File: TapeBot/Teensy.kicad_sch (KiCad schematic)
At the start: 1 part

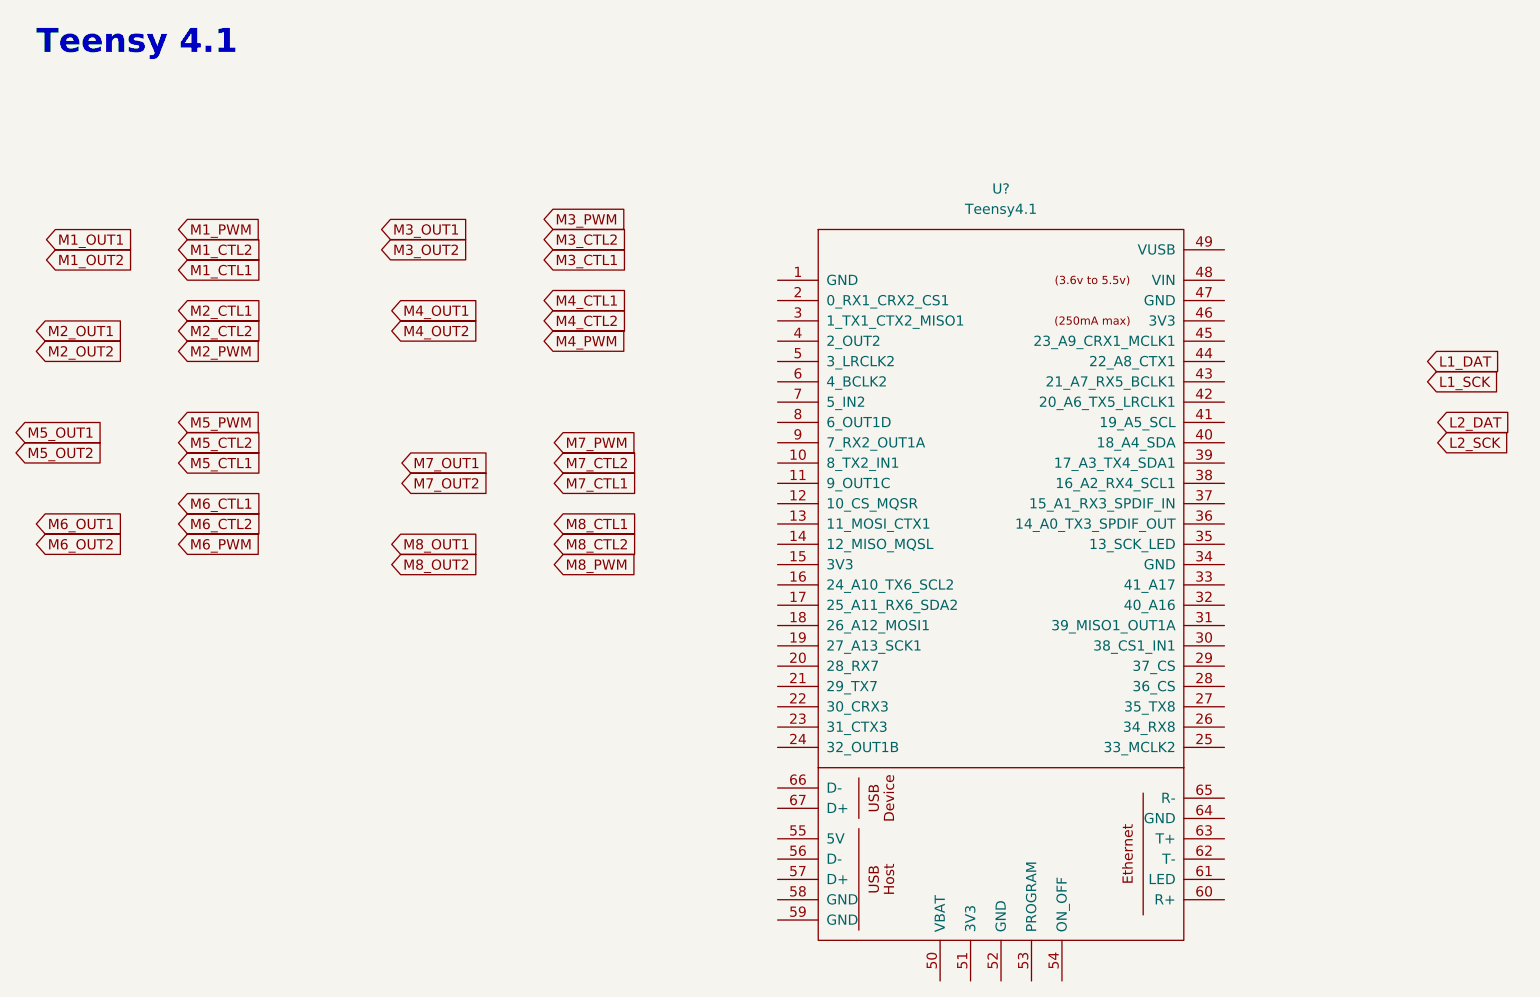
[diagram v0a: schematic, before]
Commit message: (mostly) finished schematic
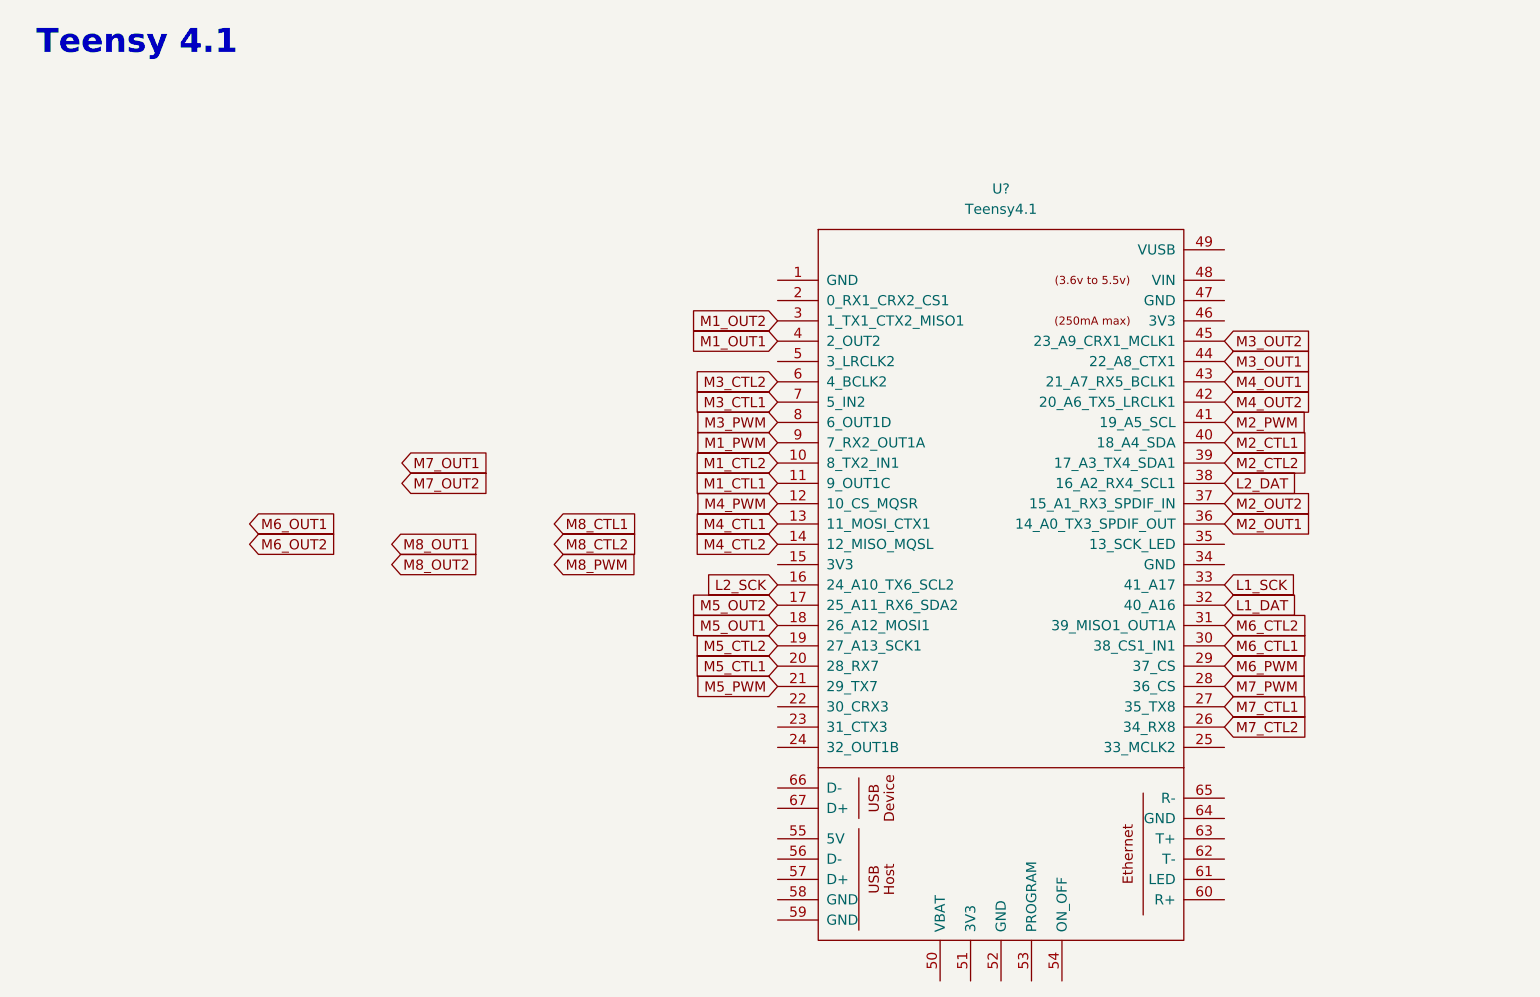
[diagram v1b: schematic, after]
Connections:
- net L1_DAT: now also U?.32 (40_A16)
- net L1_SCK: now also U?.33 (41_A17)
- net L2_DAT: now also U?.38 (16_A2_RX4_SCL1)
- net L2_SCK: now also U?.16 (24_A10_TX6_SCL2)
- net M1_CTL1: now also U?.11 (9_OUT1C)
- net M1_CTL2: now also U?.10 (8_TX2_IN1)
- net M1_OUT1: now also U?.4 (2_OUT2)
- net M1_OUT2: now also U?.3 (1_TX1_CTX2_MISO1)
- net M1_PWM: now also U?.9 (7_RX2_OUT1A)
- net M2_CTL1: now also U?.40 (18_A4_SDA)
- net M2_CTL2: now also U?.39 (17_A3_TX4_SDA1)
- net M2_OUT1: now also U?.36 (14_A0_TX3_SPDIF_OUT)
- net M2_OUT2: now also U?.37 (15_A1_RX3_SPDIF_IN)
- net M2_PWM: now also U?.41 (19_A5_SCL)
- net M3_CTL1: now also U?.7 (5_IN2)
- net M3_CTL2: now also U?.6 (4_BCLK2)
- net M3_OUT1: now also U?.44 (22_A8_CTX1)
- net M3_OUT2: now also U?.45 (23_A9_CRX1_MCLK1)
- net M3_PWM: now also U?.8 (6_OUT1D)
- net M4_CTL1: now also U?.13 (11_MOSI_CTX1)
- net M4_CTL2: now also U?.14 (12_MISO_MQSL)
- net M4_OUT1: now also U?.43 (21_A7_RX5_BCLK1)
- net M4_OUT2: now also U?.42 (20_A6_TX5_LRCLK1)
- net M4_PWM: now also U?.12 (10_CS_MQSR)
- net M5_CTL1: now also U?.20 (28_RX7)
- net M5_CTL2: now also U?.19 (27_A13_SCK1)
- net M5_OUT1: now also U?.18 (26_A12_MOSI1)
- net M5_OUT2: now also U?.17 (25_A11_RX6_SDA2)
- net M5_PWM: now also U?.21 (29_TX7)
- net M6_CTL1: now also U?.30 (38_CS1_IN1)
- net M6_CTL2: now also U?.31 (39_MISO1_OUT1A)
- net M6_PWM: now also U?.29 (37_CS)
- net M7_CTL1: now also U?.27 (35_TX8)
- net M7_CTL2: now also U?.26 (34_RX8)
- net M7_PWM: now also U?.28 (36_CS)
